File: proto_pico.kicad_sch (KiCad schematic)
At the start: 105 parts, among them J1 USB-C Receptacle, J11 Header_2.54mm_1x5, J16 Header_2.54mm_1x5, J2 Screw_Terminal_01x02, J3 Screw_Terminal_01x02, J4 Screw_Terminal_01x02, J6 Header_2.54mm_1x7, J8 Header_2.54mm_1x5, SW1 PTS647, SW2 PTS647, U1 CP2615, U2 USB 2.0 Hub, U3 AP2112K-3.3, U4 RP2040, U5 W25Q16JV, U6 LM4040DBZ-3, U7 DRV8835, U8 CS4344, Y1 Crystal_24MHz, Y2 Crystal_12MHz

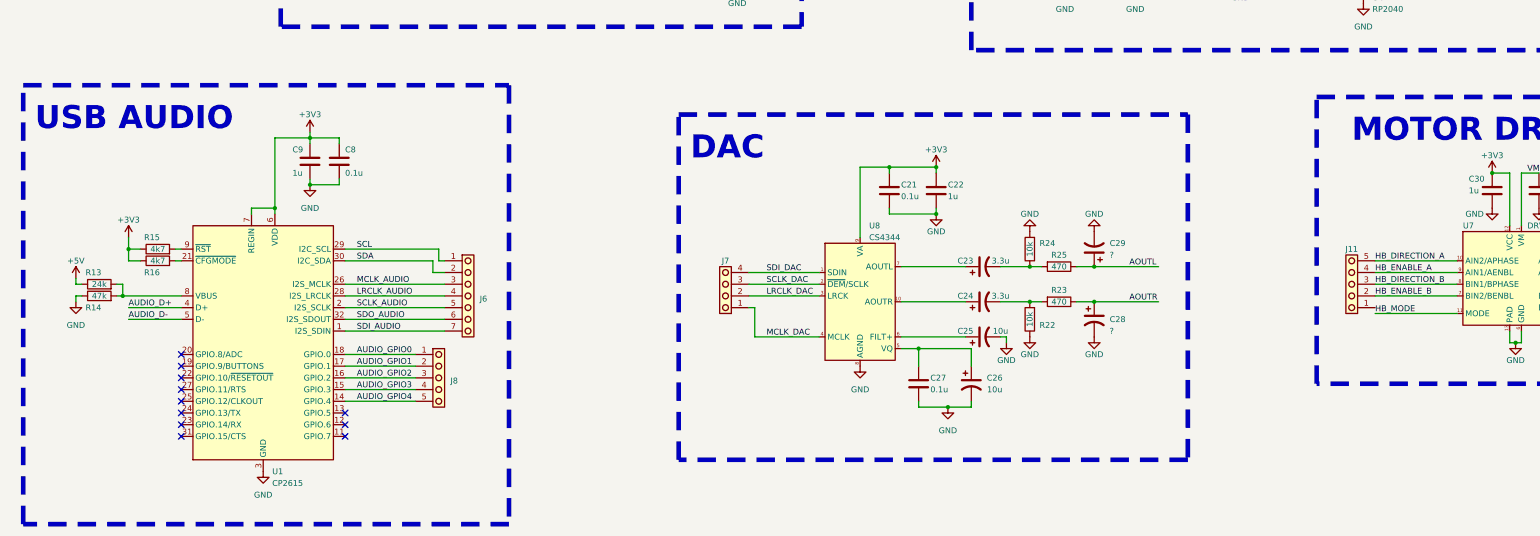
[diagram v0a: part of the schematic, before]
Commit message: done some routing
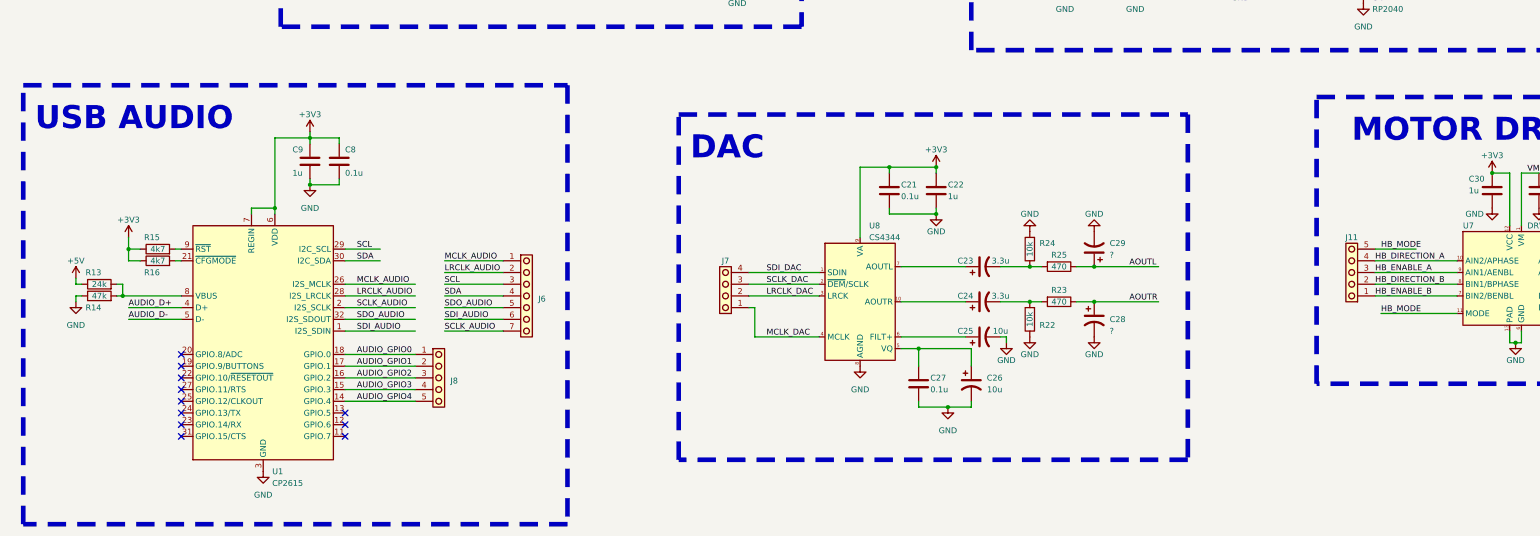
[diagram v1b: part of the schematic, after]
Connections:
- net HB_DIRECTION_A: now also J11.4; no longer J11.5
- net HB_DIRECTION_B: now also J11.2; no longer J11.3
- net HB_ENABLE_A: now also J11.3; no longer J11.4
- net HB_ENABLE_B: now also J11.1; no longer J11.2
- net HB_MODE: now also J11.5
- net LRCLK_AUDIO: now also J6.2; no longer J6.4
- net MCLK_AUDIO: now also J6.1; no longer J6.3
- net SCL: now also J6.3; no longer J6.1
- net SCLK_AUDIO: now also J6.7; no longer J6.5
- net SDA: now also J6.4; no longer J6.2
- net SDI_AUDIO: now also J6.6; no longer J6.7
- net SDO_AUDIO: now also J6.5; no longer J6.6
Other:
- moved on the sheet: J6

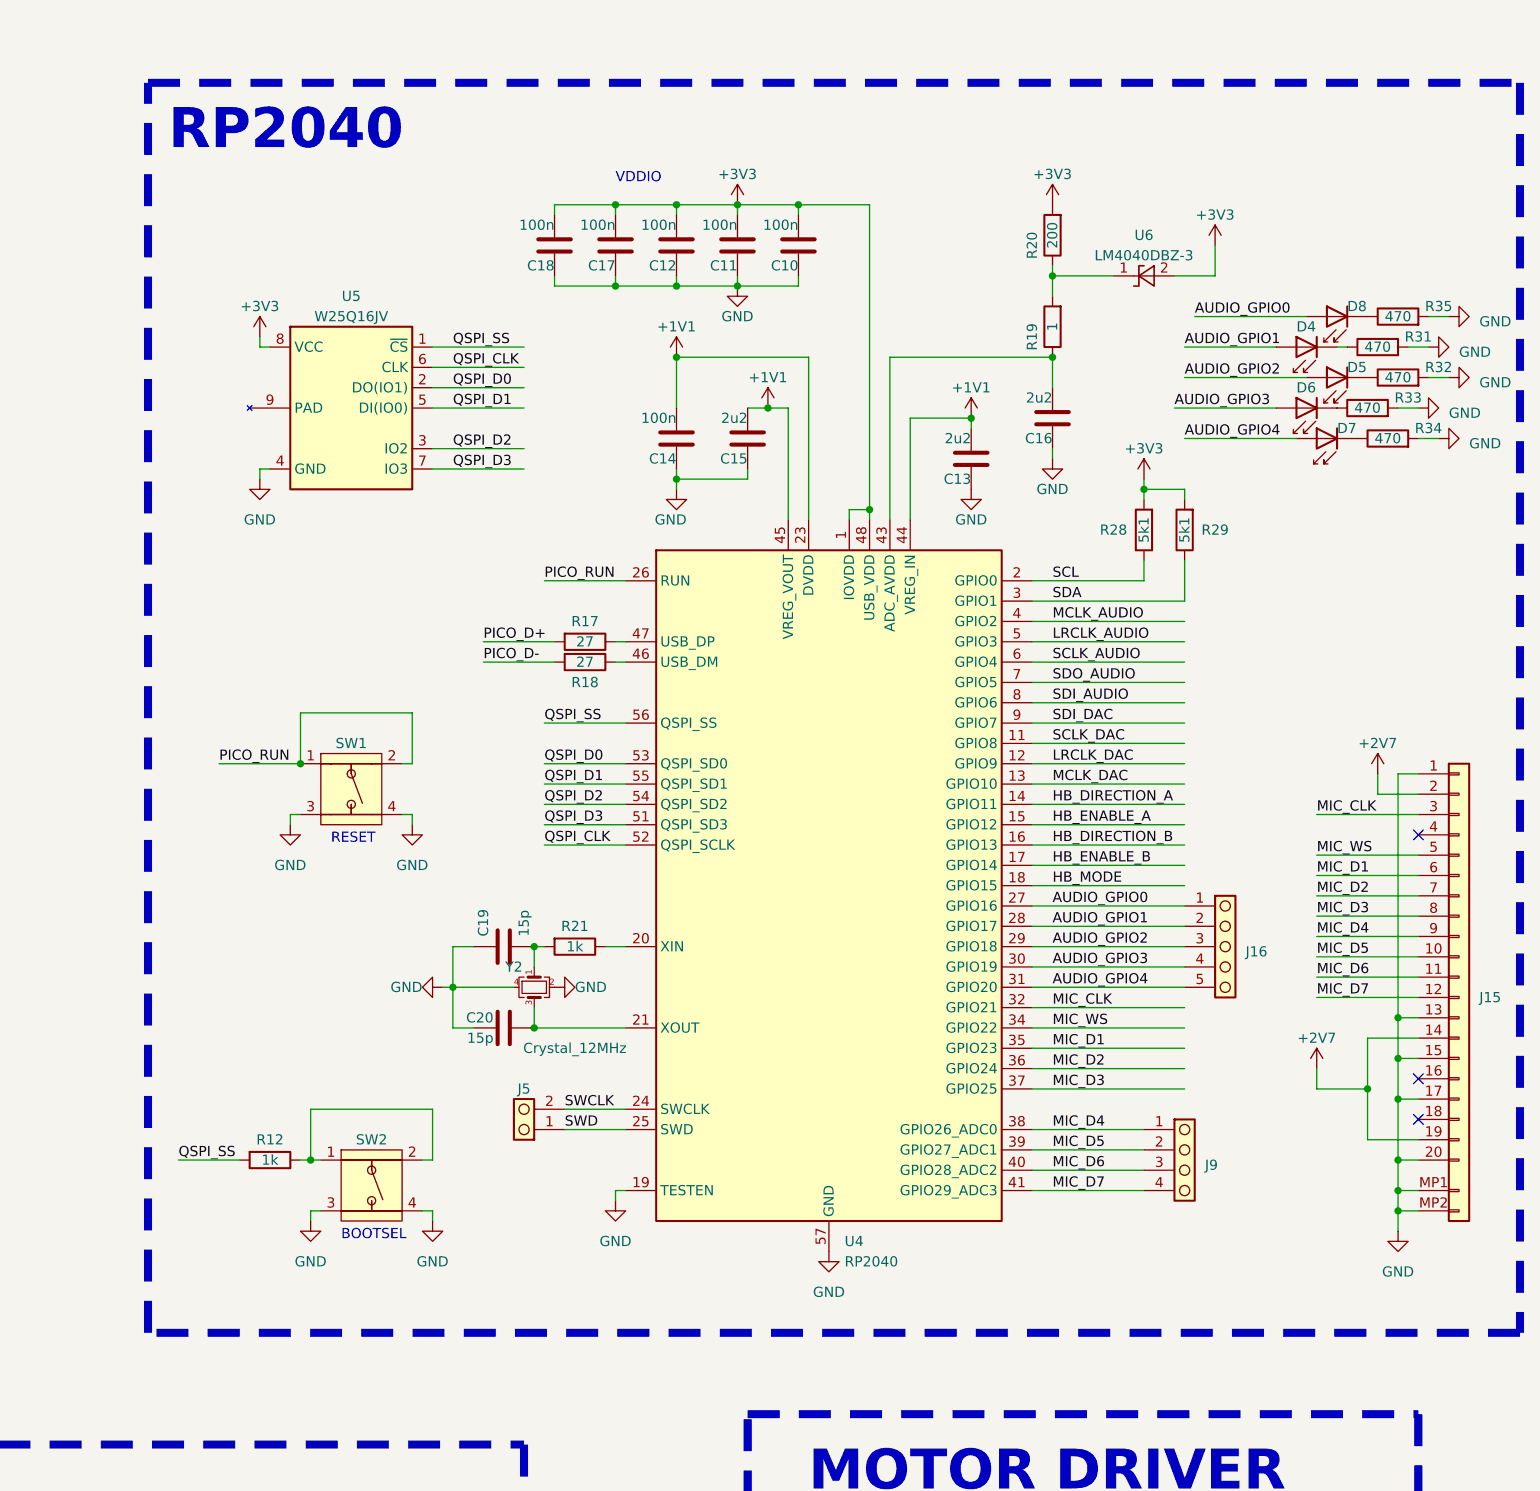
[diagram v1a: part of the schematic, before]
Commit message: some updates to schematic and component placement
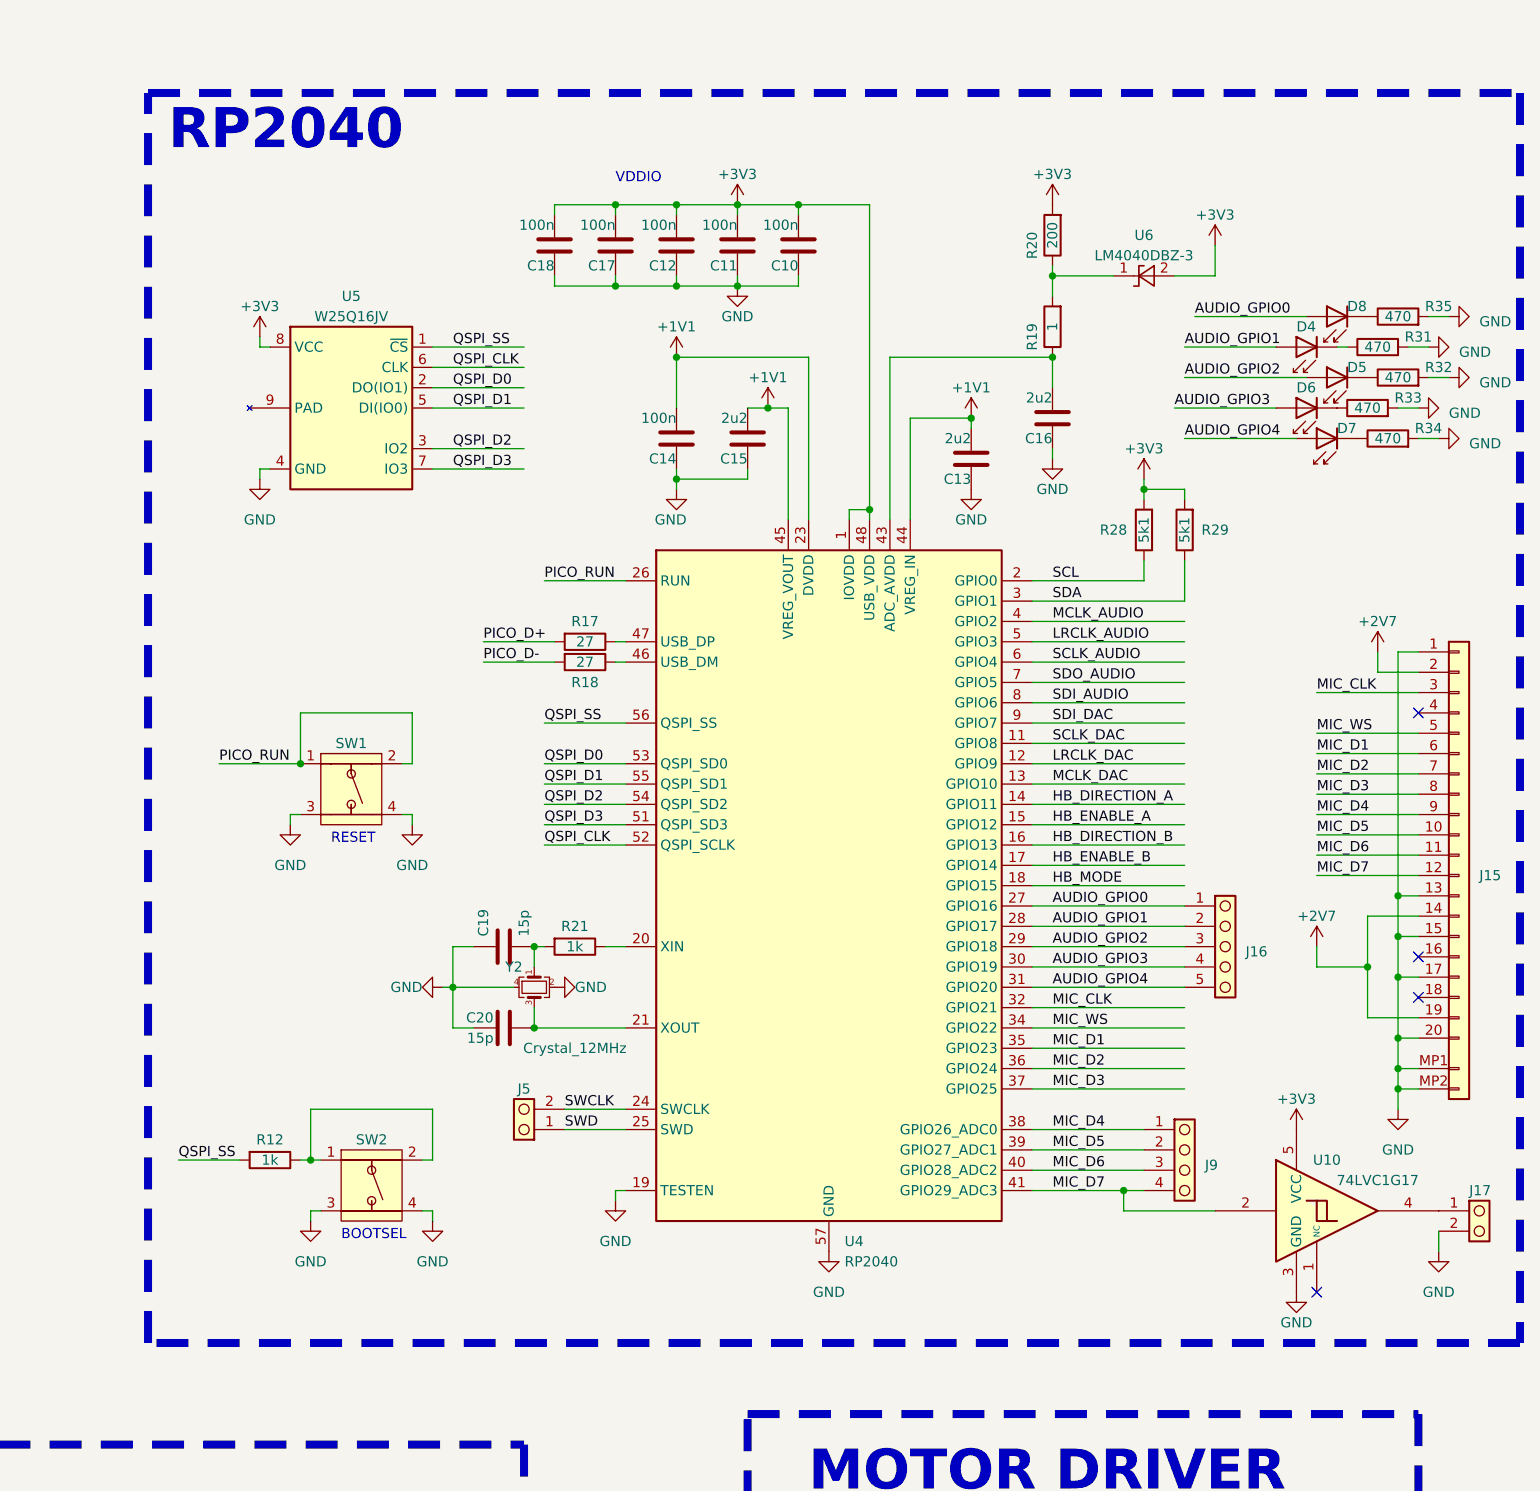
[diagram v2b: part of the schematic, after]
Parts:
- added J17: ~, Connectors:PinHeader_1x02_P2.54mm_Vertical, symbol Connectors:Header_2.54mm_1x2
- added U10: 74LVC1G17, symbol 74xGxx:74LVC1G17
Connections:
- net +3V3: now also U10.5 (VCC)
- net GND: now also J17.2 (Pin_2), U10.3 (GND)
- net MIC_D7: now also U10.2
- new net: J17.1 (Pin_1), U10.4
- no-connect marks 29 -> 30
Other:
- moved on the sheet: J15
